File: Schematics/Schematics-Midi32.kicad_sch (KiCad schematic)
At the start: 1 part

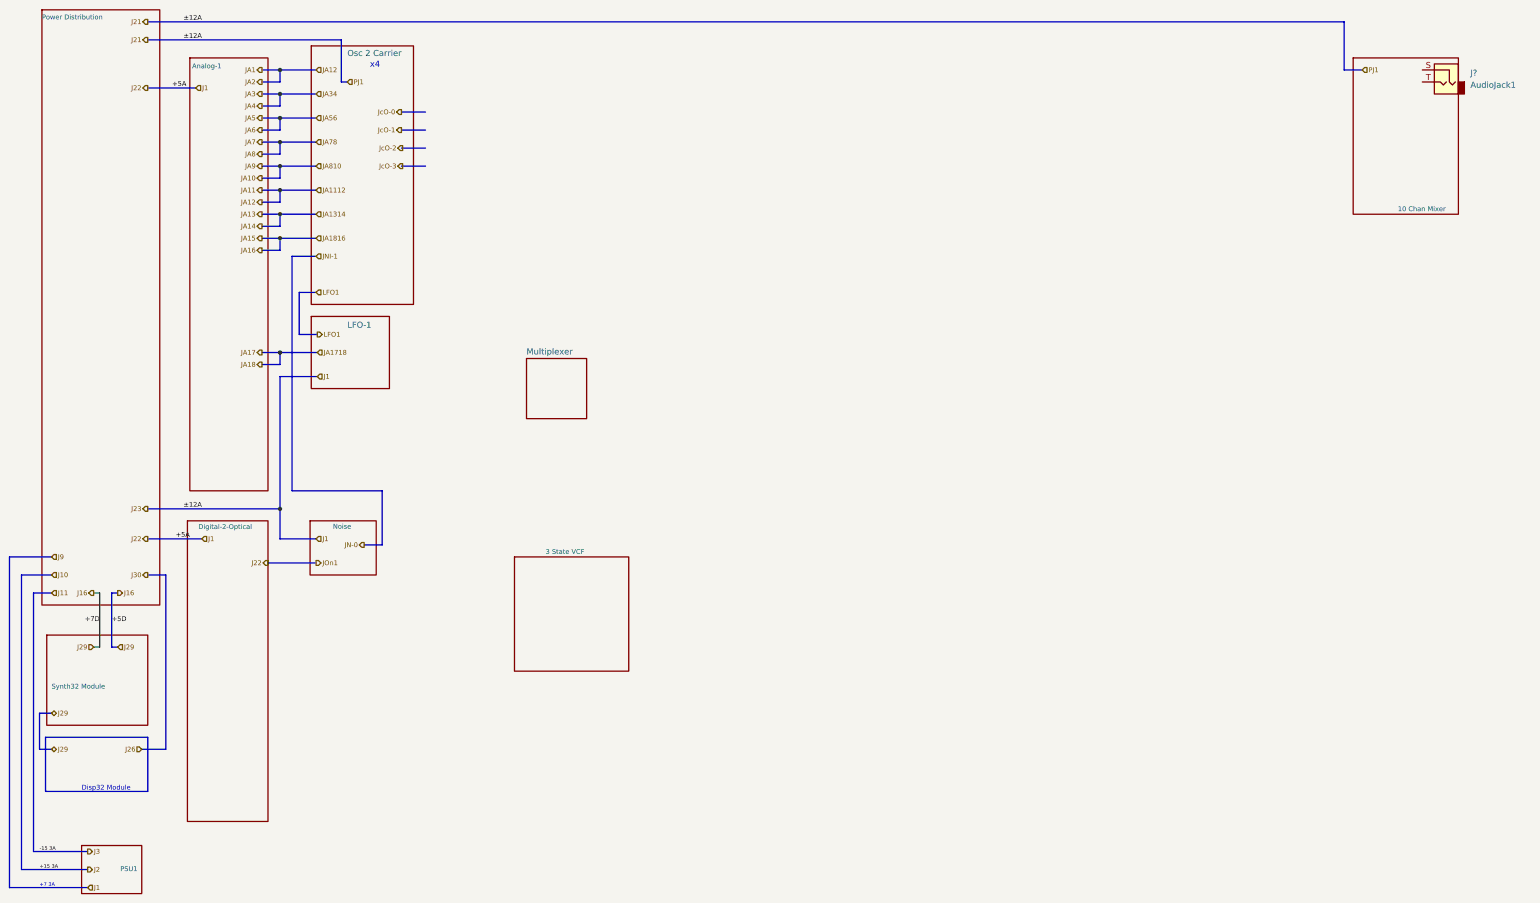
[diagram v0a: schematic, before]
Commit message: Prelude to split configurations.
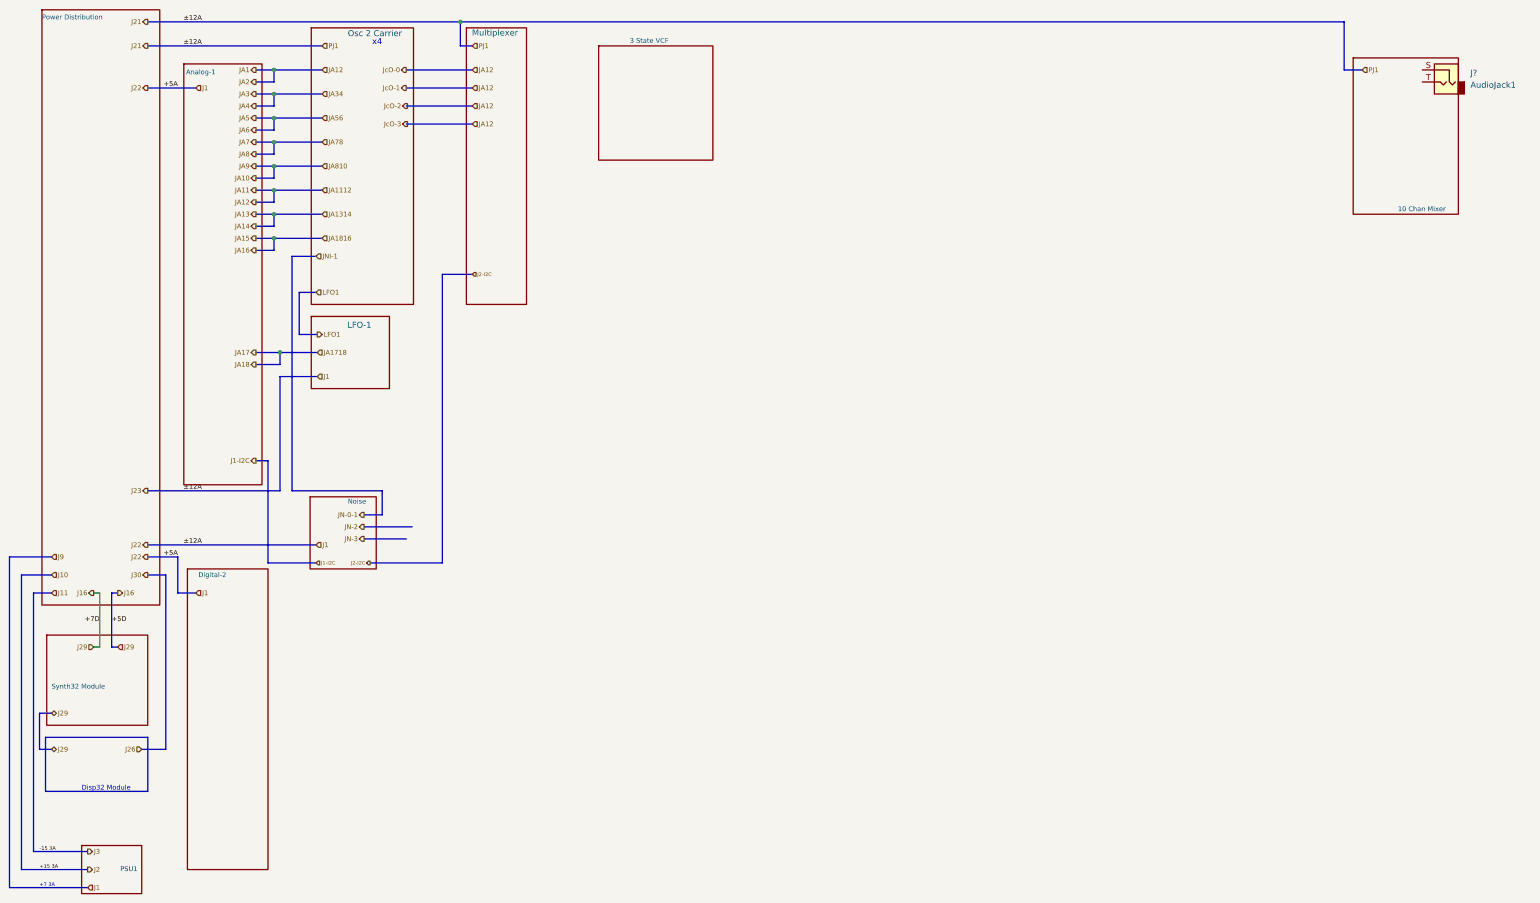
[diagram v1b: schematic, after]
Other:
- sheet Digital-2-Optical renamed Digital-2
